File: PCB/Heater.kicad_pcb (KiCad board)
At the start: 2 copper layers, 49 parts, among them IC1 ATTINY45-P, P1 220V 50Hz, P2 ICP, P3 DS18B20, U1 MOC3023M

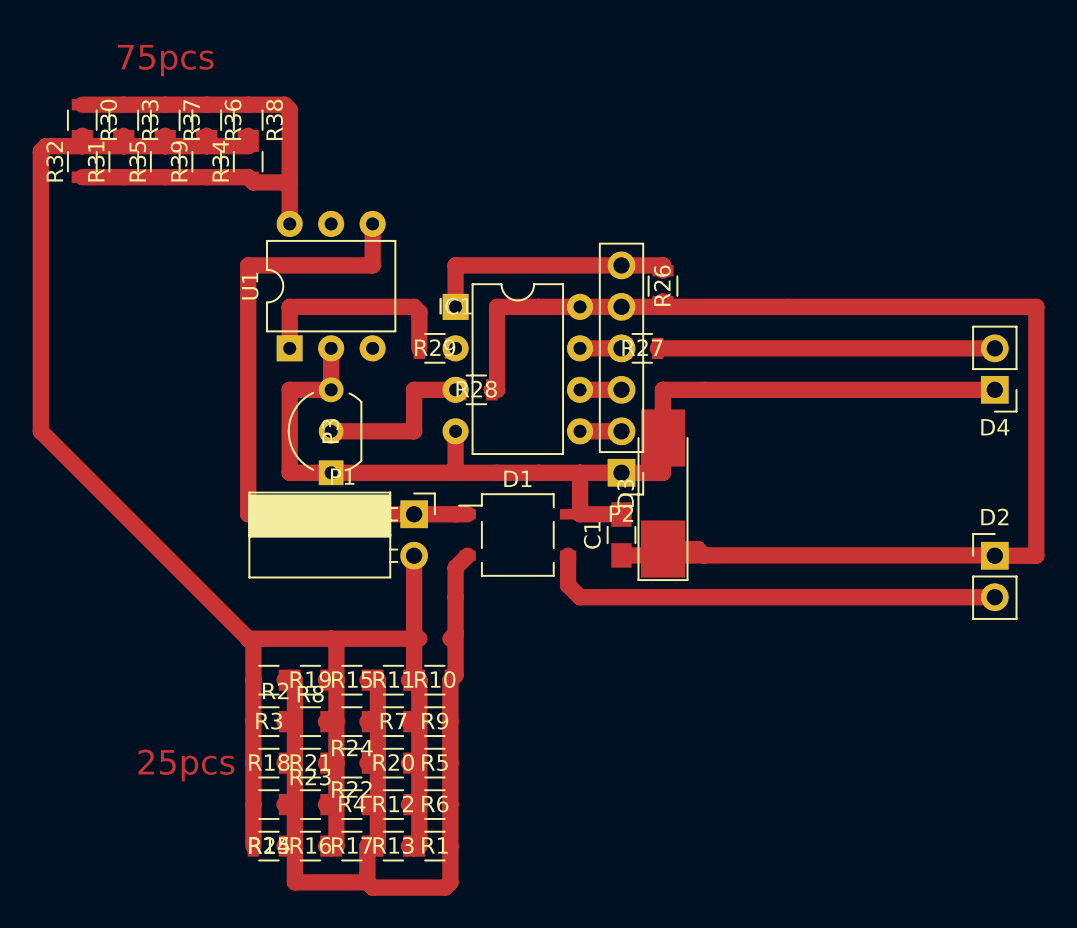
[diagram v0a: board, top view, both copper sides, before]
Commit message: Not working yet
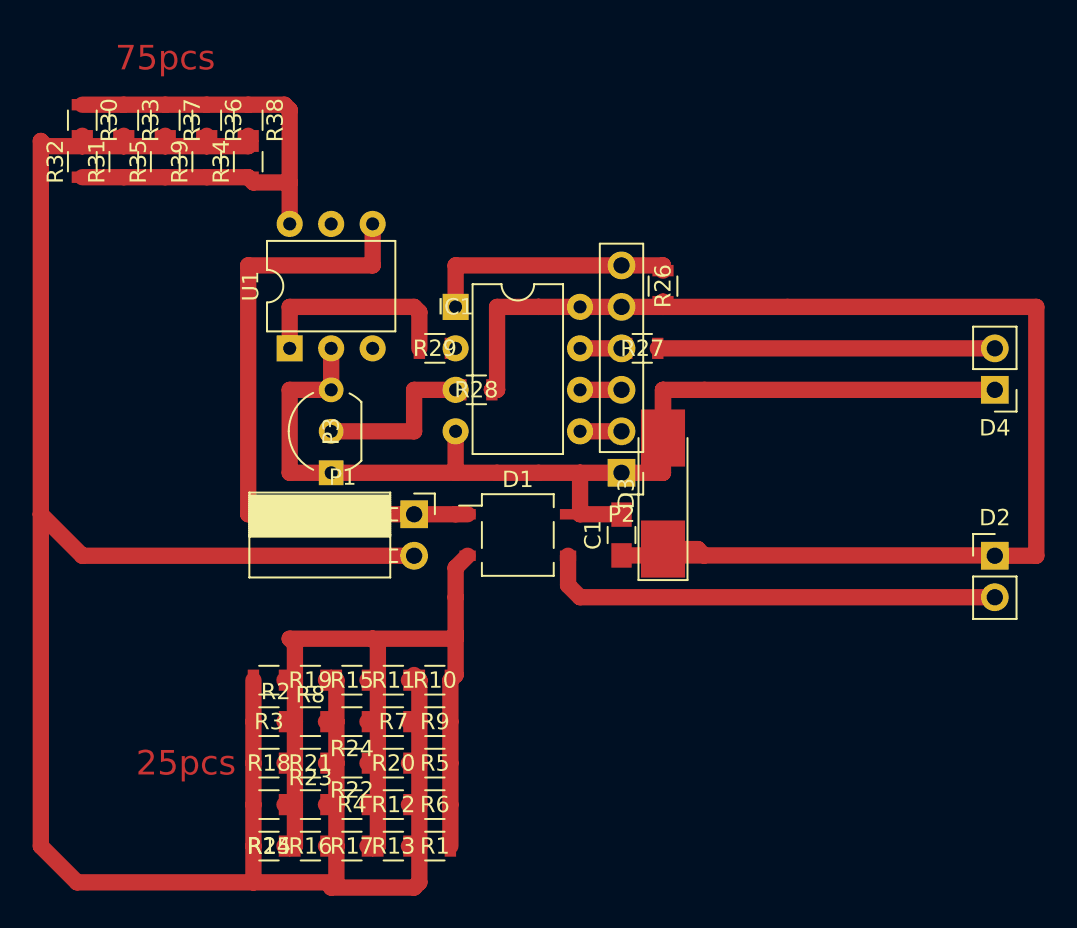
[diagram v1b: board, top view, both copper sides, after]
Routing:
- net Net-(P1-Pad2): track 112.0 -> 152.1 mm
- net Net-(D1-Pad2): track 61.8 -> 61.1 mm
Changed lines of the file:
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@@
-(kicad_pcb (version 4) (host pcbnew 4.0.4+e1-6308~48~ubuntu16.04.1-stable)
+(kicad_pcb (version 4) (host pcbnew 4.0.6-e0-6349~53~ubuntu16.04.1)
   (general
     (links 98)
     (no_connects 0)
-    (area 0 0 0 0)
+    (area 85.659999 68.65 148.020002 121.350002)
     (thickness 1.6)
     (drawings 2)
-    (tracks 156)
+    (tracks 157)
     (zones 0)
     (modules 49)
@@
     (effects (font (size 1.5 1.5) (thickness 0.3)))
   )
-  (segment (start 119.38 97.79) (end 118.645 97.79) (width 0.25) (layer F.Cu) (net 1) (status 800000))
+  (segment (start 119.38 97.79) (end 118.645 97.79) (width 0.25) (layer F.Cu) (net 1))
   (segment (start 124.46 93.12) (end 124.46 90.17) (width 1) (layer F.Cu) (net 1))
   (segment (start 119.38 97.79) (end 121.9 97.79) (width 1) (layer F.Cu) (net 1))
@@
   (segment (start 116.84 95.25) (end 119.38 95.25) (width 1) (layer F.Cu) (net 1))
   (segment (start 119.38 95.25) (end 121.92 95.25) (width 1) (layer F.Cu) (net 1))
+  (segment (start 106.68 105.41) (end 101.6 105.41) (width 1) (layer F.Cu) (net 2))
+  (segment (start 101.92 105.73) (end 101.92 107.95) (width 1) (layer F.Cu) (net 2) (status 800000))
+  (segment (start 101.6 105.41) (end 101.92 105.73) (width 1) (layer F.Cu) (net 2))
+  (segment (start 111.76 105.41) (end 106.68 105.41) (width 1) (layer F.Cu) (net 2))
+  (segment (start 107 105.73) (end 107 107.95) (width 1) (layer F.Cu) (net 2) (status 800000))
+  (segment (start 106.68 105.41) (end 107 105.73) (width 1) (layer F.Cu) (net 2))
   (segment (start 111.76 102.87) (end 111.76 101.065) (width 1) (layer F.Cu) (net 2))
-  (segment (start 111.76 105.09) (end 111.76 102.87) (width 1) (layer F.Cu) (net 2))
-  (segment (start 111.76 101.065) (end 112.495 100.33) (width 1) (layer F.Cu) (net 2) (status 800000))
+  (segment (start 111.76 105.09) (end 111.76 105.41) (width 1) (layer F.Cu) (net 2))
+  (segment (start 111.76 105.41) (end 111.76 102.87) (width 1) (layer F.Cu) (net 2))
+  (segment (start 111.76 101.065) (end 112.495 100.33) (width 1) (layer F.Cu) (net 2))
   (segment (start 101.92 118.11) (end 101.28 118.11) (width 1) (layer F.Cu) (net 2))
   (segment (start 101.92 115.57) (end 101.28 115.57) (width 1) (layer F.Cu) (net 2))
@@
   (segment (start 101.92 110.49) (end 101.28 110.49) (width 1) (layer F.Cu) (net 2))
   (segment (start 101.92 107.95) (end 101.28 107.95) (width 1) (layer F.Cu) (net 2))
-  (segment (start 106.36 120.33) (end 101.92 120.33) (width 1) (layer F.Cu) (net 2))
-  (segment (start 101.92 120.33) (end 101.92 118.11) (width 1) (layer F.Cu) (net 2))
-  (segment (start 111.44 118.11) (end 111.44 120.33) (width 1) (layer F.Cu) (net 2))
-  (segment (start 106.36 120.33) (end 106.36 118.11) (width 1) (layer F.Cu) (net 2))
-  (segment (start 106.68 120.65) (end 106.36 120.33) (width 1) (layer F.Cu) (net 2))
-  (segment (start 111.12 120.65) (end 106.68 120.65) (width 1) (layer F.Cu) (net 2))
-  (segment (start 111.44 120.33) (end 111.12 120.65) (width 1) (layer F.Cu) (net 2))
   (segment (start 101.92 110.49) (end 101.92 107.95) (width 1) (layer F.Cu) (net 2))
   (segment (start 101.92 113.03) (end 101.92 110.49) (width 1) (layer F.Cu) (net 2))
@@
   (segment (start 111.76 105.09) (end 111.76 107.63) (width 1) (layer F.Cu) (net 2))
   (segment (start 111.76 107.63) (end 111.44 107.95) (width 1) (layer F.Cu) (net 2))
-  (segment (start 111.76 105.09) (end 111.44 105.41) (width 1) (layer F.Cu) (net 2))
-  (segment (start 118.645 100.33) (end 118.645 102.135) (width 1) (layer F.Cu) (net 3) (status 400000))
+  (segment (start 118.645 100.33) (end 118.645 102.135) (width 1) (layer F.Cu) (net 3))
   (segment (start 119.38 102.87) (end 144.78 102.87) (width 1) (layer F.Cu) (net 3))
   (segment (start 118.645 102.135) (end 119.38 102.87) (width 1) (layer F.Cu) (net 3))
@@
   (segment (start 119.38 85.09) (end 121.92 85.09) (width 1) (layer F.Cu) (net 10))
   (segment (start 124.14 87.63) (end 144.78 87.63) (width 1) (layer F.Cu) (net 11))
+  (segment (start 86.36 97.79) (end 86.36 118.11) (width 1) (layer F.Cu) (net 12))
+  (segment (start 88.58 120.33) (end 99.38 120.33) (width 1) (layer F.Cu) (net 12))
+  (segment (start 86.36 118.11) (end 88.58 120.33) (width 1) (layer F.Cu) (net 12))
+  (segment (start 109.22 100.33) (end 88.9 100.33) (width 1) (layer F.Cu) (net 12) (status 400000))
+  (segment (start 86.68 75.25) (end 88.9 75.25) (width 1) (layer F.Cu) (net 12) (status 800000))
+  (segment (start 86.36 74.93) (end 86.68 75.25) (width 1) (layer F.Cu) (net 12))
+  (segment (start 86.36 97.79) (end 86.36 74.93) (width 1) (layer F.Cu) (net 12))
+  (segment (start 88.9 100.33) (end 86.36 97.79) (width 1) (layer F.Cu) (net 12))
+  (segment (start 104.46 120.33) (end 99.38 120.33) (width 1) (layer F.Cu) (net 12))
+  (segment (start 99.38 120.33) (end 99.38 118.11) (width 1) (layer F.Cu) (net 12) (status 800000))
+  (segment (start 109.54 118.11) (end 109.54 120.33) (width 1) (layer F.Cu) (net 12) (status 400000))
+  (segment (start 104.46 120.33) (end 104.46 118.11) (width 1) (layer F.Cu) (net 12) (status 800000))
+  (segment (start 104.14 120.65) (end 104.46 120.33) (width 1) (layer F.Cu) (net 12))
+  (segment (start 109.22 120.65) (end 104.14 120.65) (width 1) (layer F.Cu) (net 12))
+  (segment (start 109.54 120.33) (end 109.22 120.65) (width 1) (layer F.Cu) (net 12))
   (segment (start 88.9 75.25) (end 88.9 74.61) (width 1) (layer F.Cu) (net 12))
   (segment (start 91.44 75.25) (end 91.44 74.61) (width 1) (layer F.Cu) (net 12))
@@
   (segment (start 96.52 75.25) (end 96.52 74.61) (width 1) (layer F.Cu) (net 12))
   (segment (start 99.06 75.25) (end 99.06 74.61) (width 1) (layer F.Cu) (net 12))
-  (segment (start 88.9 75.25) (end 86.68 75.25) (width 1) (layer F.Cu) (net 12))
-  (segment (start 86.36 92.71) (end 99.38 105.73) (width 1) (layer F.Cu) (net 12))
-  (segment (start 86.36 75.57) (end 86.36 92.71) (width 1) (layer F.Cu) (net 12))
-  (segment (start 86.68 75.25) (end 86.36 75.57) (width 1) (layer F.Cu) (net 12))
-  (segment (start 104.14 105.41) (end 99.06 105.41) (width 1) (layer F.Cu) (net 12))
-  (segment (start 99.06 105.41) (end 99.38 105.73) (width 1) (layer F.Cu) (net 12))
-  (segment (start 99.38 105.73) (end 99.38 107.95) (width 1) (layer F.Cu) (net 12))
-  (segment (start 109.22 105.41) (end 104.14 105.41) (width 1) (layer F.Cu) (net 12))
-  (segment (start 104.46 105.73) (end 104.46 107.95) (width 1) (layer F.Cu) (net 12))
-  (segment (start 104.14 105.41) (end 104.46 105.73) (width 1) (layer F.Cu) (net 12))
   (segment (start 99.38 115.57) (end 99.38 118.11) (width 1) (layer F.Cu) (net 12))
   (segment (start 99.38 113.03) (end 99.38 115.57) (width 1) (layer F.Cu) (net 12))
@@
   (segment (start 104.46 115.57) (end 104.46 113.03) (width 1) (layer F.Cu) (net 12))
   (segment (start 104.46 118.11) (end 104.46 115.57) (width 1) (layer F.Cu) (net 12))
-  (segment (start 109.22 105.41) (end 109.22 107.63) (width 1) (layer F.Cu) (net 12))
   (segment (start 109.22 107.63) (end 109.54 107.95) (width 1) (layer F.Cu) (net 12))
-  (segment (start 109.22 105.41) (end 109.54 105.41) (width 1) (layer F.Cu) (net 12))
   (segment (start 109.54 110.49) (end 109.54 107.95) (width 1) (layer F.Cu) (net 12))
   (segment (start 109.54 113.03) (end 109.54 110.49) (width 1) (layer F.Cu) (net 12))
   (segment (start 109.54 115.57) (end 109.54 113.03) (width 1) (layer F.Cu) (net 12))
   (segment (start 109.54 118.11) (end 109.54 115.57) (width 1) (layer F.Cu) (net 12))
-  (segment (start 109.22 100.33) (end 109.22 105.41) (width 1) (layer F.Cu) (net 12))
   (segment (start 109.54 87.63) (end 109.54 85.41) (width 1) (layer F.Cu) (net 13))
   (segment (start 101.6 85.09) (end 101.6 87.63) (width 1) (layer F.Cu) (net 13))
@@
   (segment (start 101.6 77.47) (end 99.38 77.47) (width 1) (layer F.Cu) (net 14))
   (segment (start 99.38 77.47) (end 99.06 77.15) (width 1) (layer F.Cu) (net 14))
-  (segment (start 112.495 97.79) (end 111.76 97.79) (width 1) (layer F.Cu) (net 15) (status 400000))
+  (segment (start 112.495 97.79) (end 111.76 97.79) (width 1) (layer F.Cu) (net 15))
   (segment (start 111.76 97.79) (end 109.22 97.79) (width 1) (layer F.Cu) (net 15))
   (segment (start 106.68 80.01) (end 106.68 82.55) (width 1) (layer F.Cu) (net 15))
